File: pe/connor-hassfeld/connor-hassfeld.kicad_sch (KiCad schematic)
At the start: 3 parts, among them J1 Connor_01x02

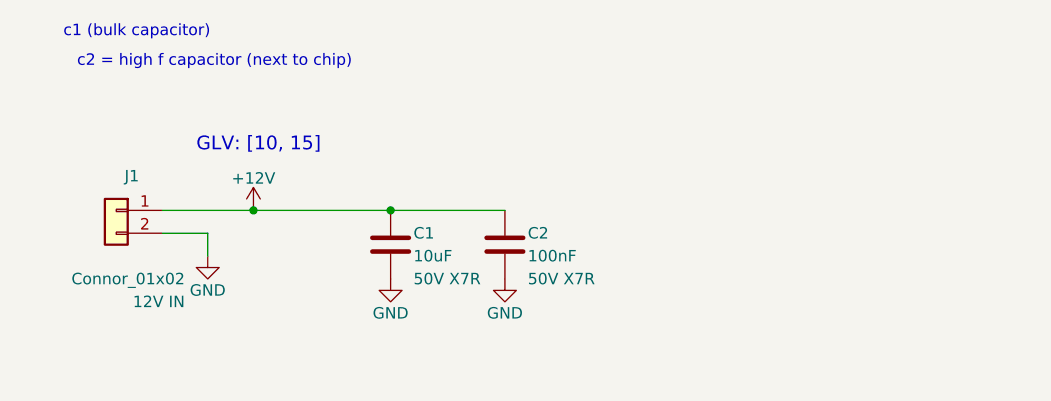
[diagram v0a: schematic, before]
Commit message: Add TPS54202 buck regulator and boot capacitor (U1, C3)
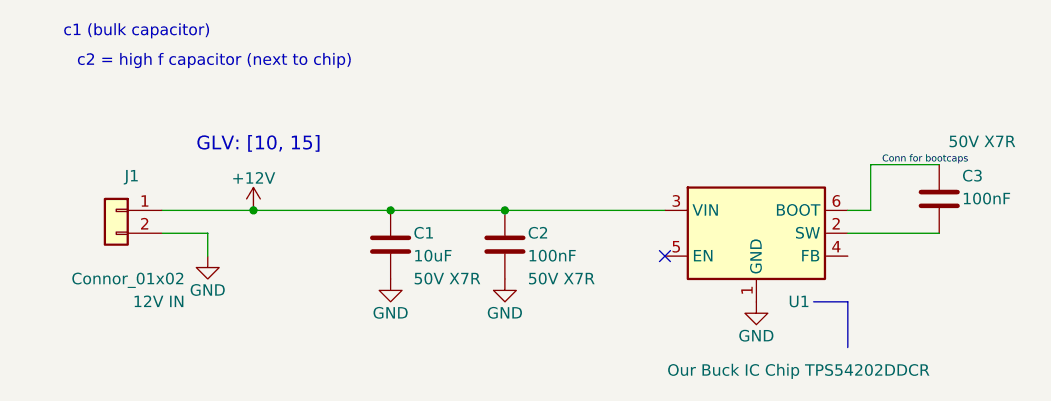
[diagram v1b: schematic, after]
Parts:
- added C3: 100nF, Capacitor_SMD:C_0603_1608Metric_Pad1.08x0.95mm_HandSolder, symbol Device:C
- added U1: Our Buck IC Chip TPS54202DDCR, Package_TO_SOT_SMD:TSOT-23-6_HandSoldering, symbol Regulator_Switching:TPS54202DDC
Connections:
- net +12V: now also U1.3 (VIN)
- net GND: now also U1.1 (GND)
- new net: C3.2, U1.2 (SW)
- new net Conn for bootcaps: C3.1, U1.6 (BOOT)
- no-connect marks 0 -> 1
